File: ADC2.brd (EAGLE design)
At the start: 99.1 x 88.9 mm, 189 parts, among them IC1 FPGA CORE BOARD, IC10 REF5040, IC11 1.8V, IC12 1.8V, IC13 2.7V, IC14 ISO6720FB, IC15 ISO6720FB, IC16 IOS6720FB, IC17 IOS6720FB, IC2 OPA, IC3 7808, IC4 LM317-L, IC5 LM337-L, IC6 LM337-L, IC7 OPA1633, IC8 AK1110, IC9 AD4134, J1 V-, J2 V-, SW1 DC, SW2 GAIN, U1 DC-DC, X1 48MHz

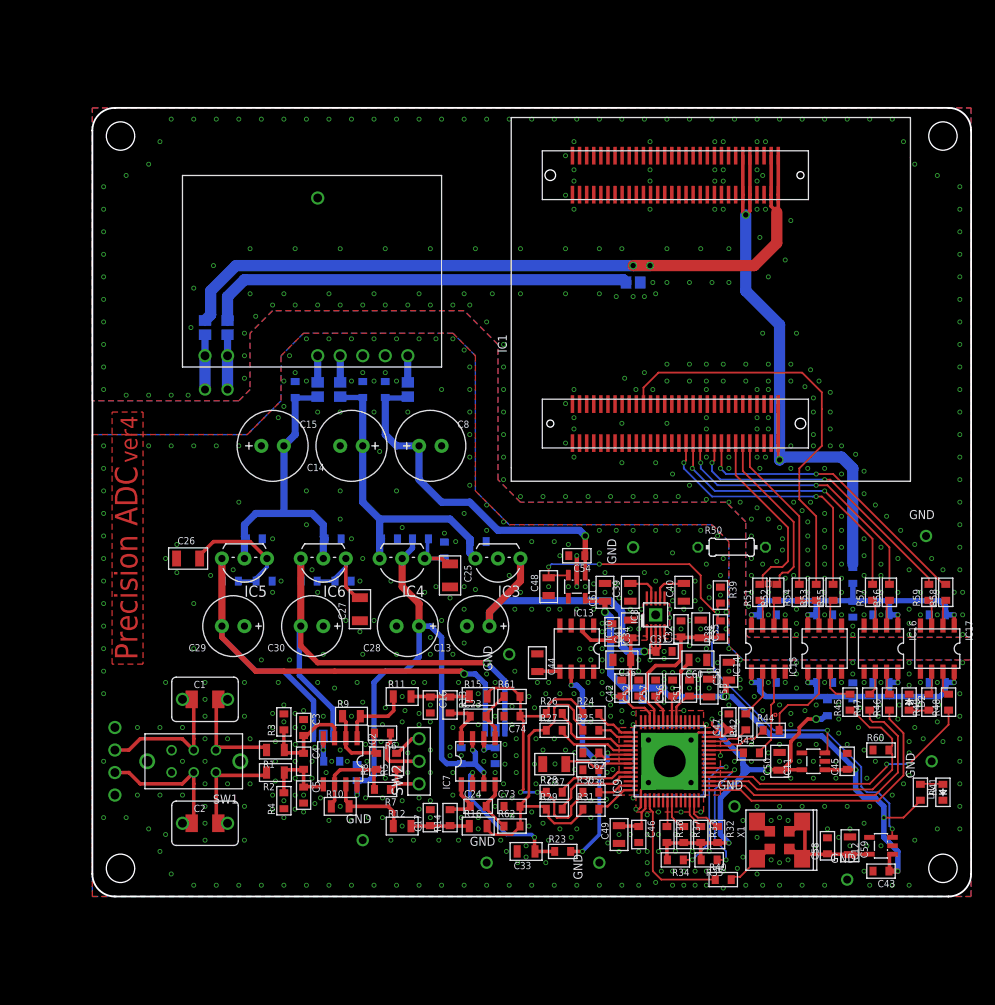
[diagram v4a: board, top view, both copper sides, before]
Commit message: 発注
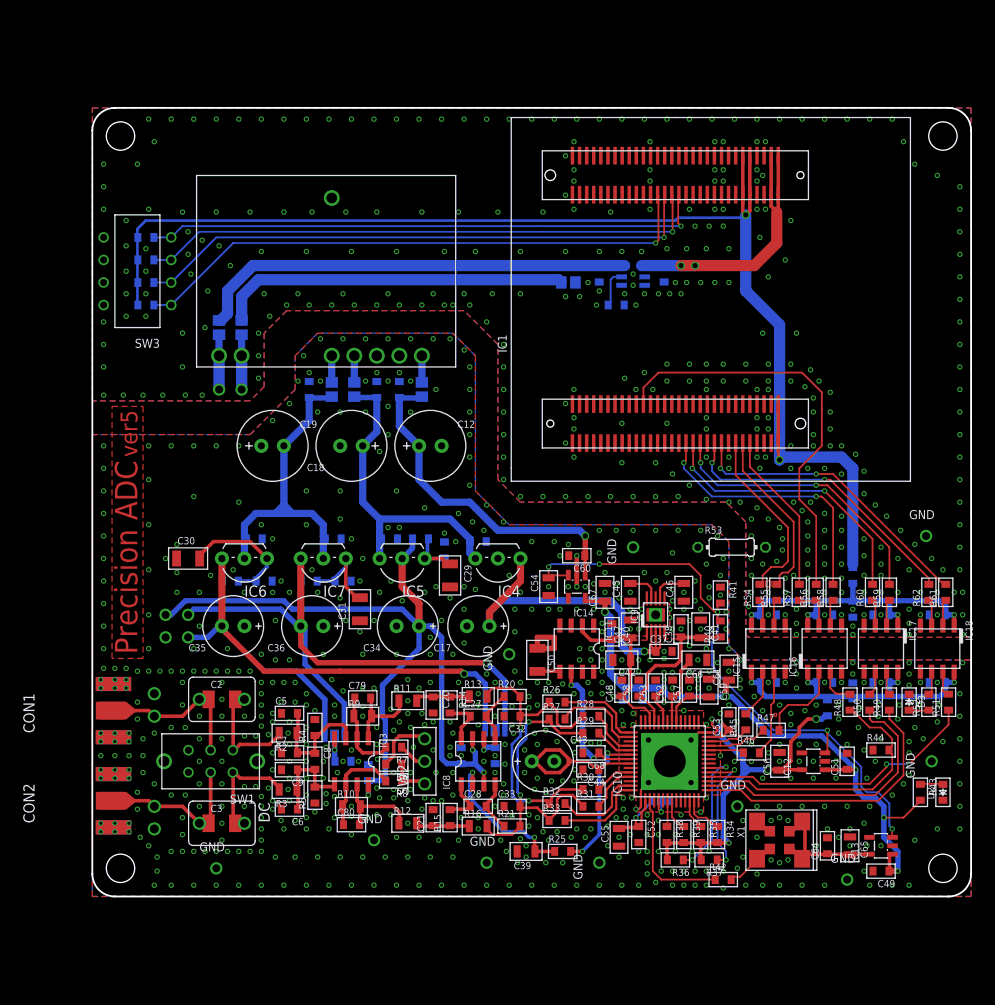
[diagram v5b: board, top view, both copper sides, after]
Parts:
- added C75, C76, C77: 0.1u, my_rcl:1608C
- added C78: 10u, my_rcl:1608C
- added C79, C80: 100p, my_rcl:1608C
- added CON1: IN-, my_connector:SMA-EDGE
- added CON2: IN+, my_connector:SMA-EDGE
- added IC18: IOS6720FB, my_ic:SOP8-2
- added J3: CLKSEL, my_rcl:1608-3-J
- added R63, R64, R65, R66: 10k, my_rcl:1608
- added SW3: FSEL, my_rcl:DIPSW-4
- added TP14, TP15: GND, my_connector:TESTPIN
- added TP16: +9V, my_connector:TESTPIN
- added TP17: -9V, my_connector:TESTPIN
- added TP18: -5V, my_connector:TESTPIN
- C1: device my_rcl:C050W -> my_rcl:1608C
- C10, C62: value 1u -> 0.1u
- C11, C38, C68: value 0.1u -> 1u
- C12, C18, C19: value 0.1u -> 100u; device my_rcl:1608C -> my_rcl:E2,5-8
- C13: value 100u -> 1u; device my_rcl:E2.5-6.5 -> my_rcl:1608C
- C14: value 100u -> 1u; device my_rcl:E2,5-8 -> my_rcl:1608C
- C15: value 100u -> 0.1u; device my_rcl:E2,5-8 -> my_rcl:1608C
- C16: value 1n -> 0.1u
- C17: value 1n -> 100u; device my_rcl:1608C -> my_rcl:E2.5-6.5
- C2: value 1u -> 1.5u
- C20, C21: value 0.1u -> 1n
- C23, C24: value 270p -> 0.1u
- C25, C26: value 10u -> 0.1u; device my_rcl:3216 -> my_rcl:1608C
- C27: value 10u -> 270p; device my_rcl:3216 -> my_rcl:1608C
- C28: value 100u -> 270p; device my_rcl:E2.5-6.5 -> my_rcl:1608C
- C29, C30: value 100u -> 10u; device my_rcl:E2.5-6.5 -> my_rcl:3216
- C3: value DNP -> 1.5u; device my_rcl:1608C -> my_rcl:C050W
- C31: value 1u -> 10u; device my_rcl:1608C -> my_rcl:3216
- C32: value 1u -> 68p
- C33: value 10u -> 68p; device my_rcl:2012 -> my_rcl:1608C
- C34: value 1u -> 100u; device my_rcl:1608C -> my_rcl:E2.5-6.5
- C35, C36: value 10u -> 100u; device my_rcl:2012 -> my_rcl:E2.5-6.5
- C37: value 10u -> 1u; device my_rcl:3216 -> my_rcl:1608C
- C4: value DNP -> 1u
- C40: value 10u -> 1u; device my_rcl:2012 -> my_rcl:1608C
- C42, C45, C46, C47, C54, C56, C65, C66, C67: value 0.1u -> 10u; device my_rcl:1608C -> my_rcl:2012
- C43: value 0.1u -> 330u; device my_rcl:1608C -> my_rcl:E2.5-6.5
- C44, C48, C49, C53, C60: value 10u -> 0.1u; device my_rcl:2012 -> my_rcl:1608C
- C50: device my_rcl:2012 -> my_rcl:3216
- C55: value 10u -> 2.2u
- C6: value 0.1u -> DNP
- C63, C72: value 10u -> 0.1u
- C69: value 0.1u -> 10u
- C7, C9: value 1u -> DNP
- C73, C74: value 47p -> 0.1u
- C8: value 100u -> DNP; device my_rcl:E2,5-8 -> my_rcl:1608C
- D1: value PWR -> TVS; device my_rcl:D1608 -> my_rcl:SOD323
- D2: value LED -> PWR
- D3: value TVS -> CLIP; device my_rcl:SOD323 -> my_rcl:D1608
- IC10: value REF5040 -> AD4134; device my_ic:SOP8 -> my_ic:QFN56-HT-HOLE
- IC11: value 1.8V -> REF5040; device my_ic:SOT23-5 -> my_ic:SOP8
- IC13: value 2.7V -> 1.8V
- IC14: value ISO6720FB -> 2.7V; device my_ic:SOP8 -> my_ic:SOT23-5
- IC15, IC17: device my_ic:SOP8 -> my_ic:SOP8-2
- IC16: value IOS6720FB -> ISO6720FB; device my_ic:SOP8 -> my_ic:SOP8-2
- IC2: value OPA -> AP22652; device my_ic:SOP8 -> my_ic:SOT23-6
- IC3: value 7808 -> OPA; device my_ic:TO-92 -> my_ic:SOP8
- IC4: value LM317-L -> 7808
- IC5: value LM337-L -> LM317-L
- IC7: value OPA1633 -> LM337-L; device my_ic:SOP8 -> my_ic:TO-92
- IC8: value AK1110 -> OPA1633; device my_ic:PLP10 -> my_ic:SOP8
- IC9: value AD4134 -> AK1110; device my_ic:QFN56-HT-HOLE -> my_ic:PLP10
- R1: value 10 -> 10k; device my_rcl:2012 -> my_rcl:1608
- R10, R9: value 1k -> 270
- R11, R12, R16: value 1k -> 510
- R13: value 360 -> 510; device my_rcl:1608 -> my_rcl:2012
- R14: value 360 -> 100
- R15: value 1k -> 100; device my_rcl:2012 -> my_rcl:1608
- R2: value 10 -> 20
- R20, R21: value 120 -> 51
- R24, R25: value 22 -> 120
- R26, R28, R29, R30, R31: value 22 -> 10; device my_rcl:1608 -> my_rcl:1608-3
- R27: value 22 -> 10
- R3: value 100k -> 20; device my_rcl:1608 -> my_rcl:2012
- R32: value 10k -> 10
- R33: value 10k -> 10; device my_rcl:1608 -> my_rcl:1608-3
- R38, R39: value 47k -> 10k
- R40: value 39 -> 47k
- R41: value 5.1k -> 47k
- R42: value ODR -> 39
- R43, R52: value DOUT -> 3.3k
- R44: value DCLK -> 10k
- R45: value SDO -> ODR
- R46: value CS -> DOUT
- R47, R57: value SCLK -> DCLK
- R48, R58: value SDI -> SDO
- R49, R59: value LED -> CS
- R5: value 360 -> 100k
- R50: value 10M -> SCLK; device my_rcl:0204/7 -> my_rcl:1608
- R51: value ODR -> SDI
- R53: value SUB -> 10M; device my_rcl:1608 -> my_rcl:0204/7
- R54: value DCLK -> ODR
- R55: value SDO -> DOUT
- R56: value CS -> SUB
- R6: value 10 -> 100
- R60: value 10k -> SCLK
- R61: value 50 -> SDI
- R62: value 50 -> LED
- R7: value 10 -> 24
- R8: value 10k -> 24
- SW1: value DC -> AC
- SW2: value GAIN -> GAIN H<>M
- moved C1 70.5 mm to (64.5, 70.2), flipped to the bottom, turned to 270 degrees
- moved C4 64.3 mm to (57.1, 70.2), flipped to the bottom
- moved IC2 63.8 mm to (61.0, 69.8), flipped to the bottom, turned to 270 degrees
- moved R1 63.2 mm to (59.1, 66.7), flipped to the bottom
- moved R62 53.9 mm to (94.3, 34.3), turned to 90 degrees
- moved C35 52.7 mm to (15.9, 30.5), turned to 180 degrees
- moved R61 50.3 mm to (96.2, 34.3), turned to 90 degrees
- moved C73 49.9 mm to (95.2, 24.1), flipped to the bottom
- moved R23 48.3 mm to (15.6, 35.6), flipped to the bottom
- moved IC13 45.0 mm to (88.9, 5.71), turned to 90 degrees
- moved C9 43.7 mm to (22.2, 14.3), flipped to the top, turned to 180 degrees
- moved C11 43.4 mm to (34.6, 57.1)
- moved C7 42.4 mm to (22.2, 16.2), flipped to the top, turned to 0 degrees
- moved R21 42.1 mm to (47.3, 7.94), flipped to the top
- moved C26 41.1 mm to (45.4, 15.9), flipped to the bottom, turned to 90 degrees
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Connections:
- removed net N$17 (its old number): IC14.6, R52.1
- new net DIPSW1: IC1.86, R63.1, SW3.1
- new net DIPSW2: IC1.88, R64.1, SW3.2
- new net DIPSW3: IC1.90, R65.1, SW3.3
- new net DIPSW4: IC1.92, R66.1, SW3.4
- new net N$32: IC16.6, R58.1
- new net N$57: IC10.47, J3.2
- new net N$63: IC2.5, R1.2
- new net VIN_LIM: C4.1, FB2.1, IC2.6
- net +1V8: now also C53.1, C56.1, IC10.13, IC12.5, R38.2, R39.2; no longer C47.1, C50.1, IC11.5, IC9.13, R32.2, R33.2
- net +1V8_ISO: now also C69.1, C70.1, C71.1, C72.1, C73.1, IC16.1, IC18.8; no longer C63.1, C64.1, C65.1, C66.1, C67.1, IC14.1, IC16.8
- net +3.6V: now also C11.1, C12.+, C60.1, IC14.1; no longer C54.1, C7.1, C8.+, IC13.1
- net +3V3D: now also R63.2, R64.2, R65.2, R66.2
- net +3V3D_ISO: now also C74.1, C75.1, C76.1, C77.1, C78.1, IC16.8, IC18.1; no longer C68.1, C69.1, C70.1, C71.1, C72.1, IC14.8, IC16.1
- net +5V: now also C38.1, C41.1, C58.1, IC10.25, IC9.5, R40.1; no longer C32.1, C35.1, C52.1, IC8.5, IC9.25, R38.1
- net +5V_DEL: now also C54.1, IC14.3, R40.2, R41.2; no longer C48.1, IC11.3, R38.2, R39.2
- net +8V: now also C17.+, C37.1, IC4.1, IC9.2, IC9.3, IC9.4; no longer C13.+, C31.1, IC3.1, IC8.2, IC8.3, IC8.4
- net +9V: now also C15.1, C25.1, C34.+, IC3.8, IC5.2, IC8.3, IC8.7, R22.2, TP16.1; no longer C11.1, C21.1, C28.+, IC2.8, IC4.2, IC7.3, IC7.7, R20.2
- net -5V: now also C36.-, IC7.3, R24.2, TP18.1; no longer C30.-, IC6.3, R22.2
- net -9V: now also C35.-, IC6.3, R23.2, TP17.1; no longer C29.-, IC5.3, R21.2
- net ADC+: now also C32.1, R13.2, R20.2, R32.1; no longer C74.1, R15.2, R24.1, R61.2
- net ADC-: now also C33.2, R21.2, R33.1; no longer C73.2, R25.1, R62.2
- net ADC_2V7: now also C49.1, C51.1, C63.1, C67.1, IC10.23, IC13.1, IC14.5, R43.2; no longer C43.1, C45.1, C55.1, C57.1, IC11.1, IC13.5, IC9.23, R41.2
- net ADC_AVDD1V8: now also C62.1, C66.1, IC10.21; no longer C56.1, C60.1, IC9.21
- net ADC_CLKVDD: now also C52.1, C55.1, IC10.44, J3.1; no longer C46.1, C49.1, IC9.44
- net ADC_CS: now also IC10.1, R49.1; no longer IC9.1, R46.1
- net ADC_DCLK: now also IC10.11, R47.1; no longer IC9.11, R44.1
- net ADC_DOUT: now also IC10.10, R46.1; no longer IC9.10, R43.1
- net ADC_DVDD1V8: now also C57.1, C59.1, IC10.20; no longer C51.1, C53.1, IC9.20
- net ADC_ODR: now also IC10.12, R45.1; no longer IC9.12, R42.1
- net ADC_SCLK: now also IC10.2, R50.1; no longer IC9.2, R47.1
- net ADC_SDI: now also IC10.4, R51.1; no longer IC9.4, R48.1
- net ADC_SDO: now also IC10.3, R44.2, R48.1; no longer IC9.3, R45.1, R60.2
- net ADC_VCOM: now also C39.2, IC8.2, R25.1; no longer C33.2, IC7.2, R23.1
- net AVDD5V: now also C40.1, C47.1, C48.1, D1.2, IC10.26, IC11.2, IC9.1; no longer C34.1, C36.1, C41.1, D3.2, IC10.2, IC8.1, IC9.26
- net DGND: now also C1.2, C4.2, C74.2, C75.2, C76.2, C77.2, C78.2, IC16.5, IC18.4, IC2.2, IC2.3, R1.1, R53.2, SW3.5, SW3.6, SW3.7, SW3.8; no longer C68.2, C69.2, C70.2, C71.2, C72.2, IC14.5, IC16.4, R50.2
- net FPGA_CS: now also R59.2; no longer R56.2
- net FPGA_DCLK: now also R57.2; no longer R54.2
- net FPGA_DCLK_SUB: now also R56.2; no longer R53.2
- net FPGA_DOUT: now also R55.2; no longer R52.2
- net FPGA_LED: now also R62.2; no longer R59.2
- net FPGA_ODR: now also R54.2; no longer R51.2
- net FPGA_SCLK: now also R60.2; no longer R57.2
- net FPGA_SDI: now also R61.2; no longer R58.2
- net FPGA_SDO: now also R58.2; no longer R55.2
- net GND: now also C10.2, C12.-, C13.2, C14.1, C15.2, C16.1, C17.-, C18.-, C19.+, C20.2, C22.2, C23.1, C24.1, C29.2, C30.1, C31.1, C34.-, C35.+, C36.+, C39.1, C43.-, C5.1, C68.2, C69.2, C7.1, C70.2, C71.2, C72.2, C73.2, CON1.G1, CON1.G2, CON1.G3, CON1.G4, CON2.G1, CON2.G2, CON2.G3, CON2.G4, D1.1, D3.K, IC10.14, IC10.19, IC10.22, IC10.24, IC10.27, IC10.31, IC10.37, IC10.40, IC10.43, IC10.HT, IC10.HT1, IC10.HT2, IC10.HT3, IC10.HT4, IC11.4, IC14.2, IC16.4, IC18.5, IC4.2, IC9.10, IC9.6, IC9.8, J3.3, R4.2, R41.1, R44.1, R5.1, R53.1, TP14.1, TP15.1; no longer C10.1, C12.1, C13.-, C14.-, C15.+, C16.2, C17.2, C18.2, C19.1, C20.1, C22.1, C27.1, C28.-, C29.+, C3.1, C30.+, C31.2, C34.2, C35.2, C36.2, C39.2, C43.2, C5.2, C7.2, C73.1, C74.2, C8.-, D1.K, D3.1, IC10.4, IC11.2, IC14.4, IC16.5, IC3.2, IC8.10, IC8.6, IC8.8, IC8.HT, IC9.14, IC9.19, IC9.22, IC9.24, IC9.27, IC9.31, IC9.37, IC9.40, IC9.43, IC9.47, IC9.HT1, IC9.HT3, IC9.HT4, R3.2, R39.1, R4.1, R50.1, R60.1
- net N$1: now also C80.1, IC3.6, R8.2; no longer IC2.6, R7.2, R8.1
- net N$10: now also IC16.2, R47.2; no longer IC15.2, R44.2
- net N$11: now also IC10.42, R33.2; no longer IC9.42, R31.2
- net N$12: now also C80.2, IC3.7; no longer IC2.7
- net N$13: now also IC10.41, R32.2; no longer IC9.41, R30.2
- net N$14: now also C5.2, C7.2, C8.1, IC3.3, R2.2, R4.1; no longer C3.2, C4.1, IC2.3, R1.2, R3.1
- net N$15: now also IC10.39, R31.2; no longer IC9.39, R29.2
- net N$16: now also IC16.3, R48.2; no longer IC15.3, R45.2
- net N$18: now also IC10.38, R30.2; no longer IC9.38, R28.2
- net N$19: now also C21.1, R15.1; no longer C17.1, R14.1
- net N$2: now also IC10.34, R25.2; no longer IC9.34, R23.2
- net N$20: now also IC10.33, R29.2; no longer IC9.33, R27.2
- net N$21: now also IC15.7, R54.1; no longer IC14.7, R51.1
- net N$22: now also C27.2, IC8.5, R20.1; no longer C23.2, IC7.5, R61.1
- net N$23: now also C6.1, C8.2, C9.1, IC3.5, R3.2, R5.2; no longer C4.2, C5.1, IC2.5, R2.2, R4.2
- net N$24: now also C27.1, IC8.8, R14.2; no longer C23.1, IC7.8, R13.2
- net N$25: now also IC10.32, R28.2; no longer IC9.32, R26.2
- net N$26: now also C28.1, IC8.1, R15.2; no longer C24.1, IC7.1, R14.2
- net N$27: now also IC16.7, R56.1, R57.1; no longer IC15.7, R53.1, R54.1
- net N$28: now also IC10.30, R27.2; no longer IC9.30, R25.2
- net N$29: now also IC10.29, R26.2; no longer IC9.29, R24.2
- net N$3: now also C79.1, IC3.2, R7.2; no longer IC2.2, R6.2, R8.2
- net N$30: now also R42.2; no longer R40.2
- net N$31: now also C28.2, IC8.4, R21.1; no longer C24.2, IC7.4, R62.1
- net N$33: now also IC17.6, R50.2; no longer IC16.6, R47.2
- net N$34: now also IC17.7, R49.2; no longer IC16.7, R46.2
- net N$35: now also IC18.6, R52.2; no longer IC17.6, R49.2
- net N$36: now also IC18.7, R51.2; no longer IC17.7, R48.2
- net N$37: now also IC17.3, R60.1; no longer IC16.3, R57.1
- net N$38: now also IC17.2, R59.1; no longer IC16.2, R56.1
- net N$39: now also IC18.3, R62.1; no longer IC17.3, R59.1
- net N$4: now also C79.2, IC3.1; no longer IC2.1
- net N$40: now also IC18.2, R61.1; no longer IC17.2, R58.1
- net N$41: now also C2.1, C2.3, CON1.SIG; no longer C1.1, C1.3
- net N$42: now also C3.1, C3.3, CON2.SIG; no longer C2.1, C2.3
- net N$43: now also C2.2, C2.4, R2.1; no longer C1.2, C1.4, R1.1
- net N$44: now also C3.2, C3.4, R3.1; no longer C2.2, C2.4, R2.1
- net N$45: now also R7.1; no longer R6.1
- net N$46: now also R6.1, R8.1; no longer R5.1, R7.1
- net N$47: now also D3.A, R52.1; no longer D2.A, R49.1
- net N$48: now also C50.1, IC11.5; no longer C44.1, IC10.5
- net N$49: now also IC10.5, R37.1; no longer IC9.5, R35.1
- net N$5: now also C20.1, R14.1; no longer C16.1, R15.1
- net N$50: now also IC10.6, R36.1; no longer IC9.6, R34.1
- net N$52: now also C16.2, IC3.4; no longer C12.2, IC2.4
- net N$53: now also C29.1, IC5.1, R22.1; no longer C25.1, IC4.1, R20.1
- net N$54: now also C30.2, IC6.1, R23.1; no longer C26.2, IC5.1, R21.1
- net N$55: now also C31.2, IC7.1, R24.1; no longer C27.2, IC6.1, R22.1
- net N$58: now also D2.A, R43.1; no longer D1.A, R41.1
- net N$59: now also R6.2; no longer R5.2
- net N$6: now also C45.1, IC9.9; no longer C39.1, IC8.9
- net N$60: now also IC10.50, R39.1; no longer IC9.50, R37.1
- net N$61: now also IC10.55, R34.1; no longer IC9.55, R32.1
- net N$62: now also IC10.54, R35.1; no longer IC9.54, R33.1
- net N$64: now also IC10.49, R38.1; no longer IC9.49, R36.1
- net N$7: now also C46.1, IC9.7; no longer C40.1, IC8.7
- net N$74: now also C26.2, IC8.6; no longer C22.2, IC7.6
- net N$8: now also IC15.2, R45.2; no longer IC14.2, R42.2
- net N$9: now also IC15.3, R46.2; no longer IC14.3, R43.2
- net OSC_CLK: now also IC10.45, R42.1; no longer IC9.45, R40.1
- net V+: now also C10.1, C13.1, C18.+, C22.1, IC5.3; no longer C14.+, C18.1, C6.1, C9.1, IC3.3
- net V-: now also C14.2, C19.-, C23.2, C24.2, IC7.2; no longer C10.2, C15.-, C19.2, C20.2, IC5.2
- net VCC_OSC: now also C64.1, C65.1, IC13.5; no longer C58.1, C59.1, IC12.5
- net VIN: now also C1.1, IC2.1; no longer FB2.1
- net VREF: now also C68.1, IC10.35, IC11.6; no longer C62.1, IC10.6, IC9.35
- net VREFCAP: now also C43.+, C44.1, IC10.36; no longer C37.1, C38.1, IC9.36
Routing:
- net +3V3D: track 69.3 -> 147.3 mm
- net DIPSW1: track 0.00 -> 65.1 mm, vias 0 -> 1
- net DIPSW2: track 0.00 -> 64.5 mm, vias 0 -> 1
- net DIPSW3: track 0.00 -> 64.0 mm, vias 0 -> 1
- net DIPSW4: track 0.00 -> 63.7 mm, vias 0 -> 1
- net VIN: track 88.1 -> 34.9 mm
- net VIN_LIM: track 0.00 -> 50.3 mm
- net +9V: track 62.9 -> 91.7 mm
- net -5V: track 56.6 -> 70.8 mm
- net VREFCAP: track 8.13 -> 18.7 mm
- net N$56: track 48.5 -> 39.6 mm
- net N$28: track 3.90 -> 10.4 mm
- net N$13: track 3.90 -> 10.2 mm
- net N$11: track 4.48 -> 9.75 mm
- net N$29: track 4.63 -> 9.75 mm
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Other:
- board text added: "DC"
- board text added: "ver5"
- board text removed: "ver4"

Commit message: 入力回路変更
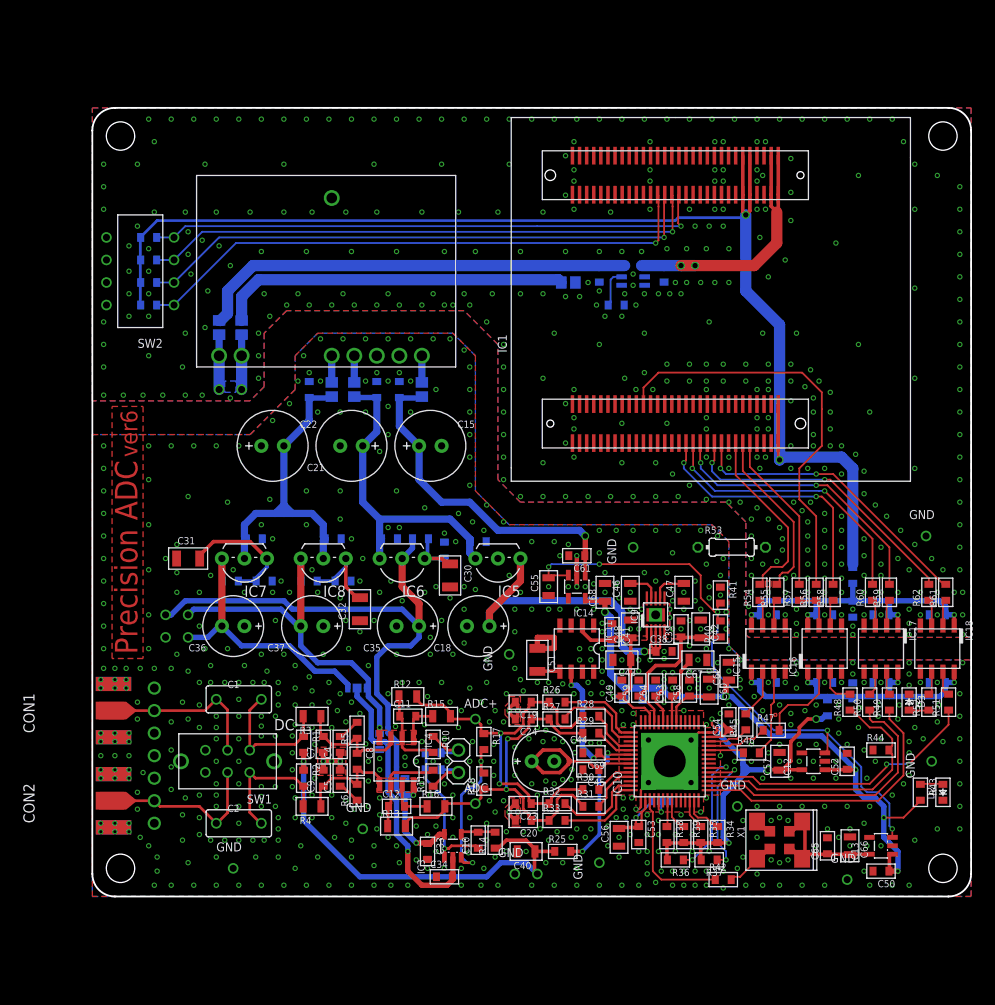
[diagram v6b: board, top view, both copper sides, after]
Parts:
- removed C80: 100p, my_rcl:1608C
- removed J3: CLKSEL, my_rcl:1608-3-J
- removed SW3: FSEL, my_rcl:DIPSW-4
- added JP1: GAIN, my_connector:1X02
- added TP19, TP20, TP21: GND, my_connector:TESTPIN-MID
- added TP22: VCOM, my_connector:TESTPIN
- added TP23: ADC+, my_connector:TESTPIN
- added TP24: ADC-, my_connector:TESTPIN
- C1: value 1u -> 1.5u; device my_rcl:1608C -> my_rcl:C050
- C10: value 0.1u -> 68p; device my_rcl:1608C -> my_rcl:1608-3
- C11: value 1u -> 100p
- C12: value 100u -> 100p; device my_rcl:E2,5-8 -> my_rcl:1608C
- C13: value 1u -> 0.1u
- C15, C22: value 0.1u -> 100u; device my_rcl:1608C -> my_rcl:E2,5-8
- C16: value 0.1u -> 1u
- C17: value 100u -> 1u; device my_rcl:E2.5-6.5 -> my_rcl:1608C
- C18: device my_rcl:E2,5-8 -> my_rcl:E2.5-6.5
- C19: value 100u -> 100p; device my_rcl:E2,5-8 -> my_rcl:1608-3
- C2: device my_rcl:C050W -> my_rcl:C050
- C20: value 1n -> 100p; device my_rcl:1608C -> my_rcl:1608-3
- C21: value 1n -> 100u; device my_rcl:1608C -> my_rcl:E2,5-8
- C23, C24: value 0.1u -> 100p
- C27, C28: value 270p -> 0.1u
- C29, C50: value 10u -> 0.1u; device my_rcl:3216 -> my_rcl:1608C
- C3: value 1.5u -> 1u; device my_rcl:C050W -> my_rcl:1608C
- C32: value 68p -> 10u; device my_rcl:1608C -> my_rcl:3216
- C33: value 68p -> 0.1u
- C34: value 100u -> 0.1u; device my_rcl:E2.5-6.5 -> my_rcl:1608C
- C37: value 1u -> 100u; device my_rcl:1608C -> my_rcl:E2.5-6.5
- C39, C41: value 10u -> 1u; device my_rcl:2012 -> my_rcl:1608C
- C4: value 1u -> 22p
- C40, C68: value 1u -> 10u; device my_rcl:1608C -> my_rcl:2012
- C43: value 330u -> 10u; device my_rcl:E2.5-6.5 -> my_rcl:2012
- C44: value 0.1u -> 330u; device my_rcl:1608C -> my_rcl:E2.5-6.5
- C45, C54, C59, C61, C65: value 10u -> 0.1u; device my_rcl:2012 -> my_rcl:1608C
- C48, C57, C60, C62: value 0.1u -> 10u; device my_rcl:1608C -> my_rcl:2012
- C5: value DNP -> 22p
- C51: value 0.1u -> 10u; device my_rcl:1608C -> my_rcl:3216
- C55: value 2.2u -> 10u
- C56: value 10u -> 2.2u
- C6: value DNP -> 1u
- C69: value 10u -> 1u
- C70: value 0.1u -> 10u
- C78: value 10u -> 0.1u
- C79: value 100p -> 10u
- C8: device my_rcl:1608C -> my_rcl:1608-3
- IC15, IC16: value ISO6720FB -> SI8620
- IC17, IC18: value IOS6720FB -> SI8620
- IC3: device my_ic:SOP8 -> my_ic:SOT23-5
- IC4: value 7808 -> OPA; device my_ic:TO-92 -> my_ic:SOP8
- IC5: value LM317-L -> 7808
- IC6: value LM337-L -> LM317-L
- IC8: value OPA1633 -> LM337-L; device my_ic:SOP8 -> my_ic:TO-92
- J1: value V- -> V-SEL; device my_rcl:2012-3-J -> my_rcl:1608-3-J
- J2: value V- -> CLKSEL; device my_rcl:2012-3-J -> my_rcl:1608-3-J
- R1: value 10k -> 100k; device my_rcl:1608 -> my_rcl:1608-3
- R10: value 270 -> 24; device my_rcl:2012 -> my_rcl:1608-3
- R11: value 510 -> 24; device my_rcl:2012 -> my_rcl:1608-3
- R12, R13, R3: device my_rcl:2012 -> my_rcl:2012-R
- R14: value 100 -> 1k
- R15: value 100 -> 270; device my_rcl:1608 -> my_rcl:2012-R
- R16: value 510 -> 270; device my_rcl:2012 -> my_rcl:2012-R
- R17, R18: value 680 -> 3.6k
- R19: value 330 -> 680
- R2: value 20 -> 100k; device my_rcl:2012 -> my_rcl:1608-3
- R20: value 51 -> 680
- R21: value 51 -> 330
- R4: value 100k -> 20; device my_rcl:1608 -> my_rcl:2012-R
- R5: value 100k -> 50; device my_rcl:1608 -> my_rcl:1608-3
- R6: value 100 -> 50; device my_rcl:1608 -> my_rcl:1608-3
- R7: value 24 -> 10k
- R8: value 24 -> 1k; device my_rcl:1608 -> my_rcl:1608-3
- R9: value 270 -> 1k; device my_rcl:2012 -> my_rcl:1608-3
- SW2: value GAIN H<>M -> MODE-SW; device my_connector:1X03 -> my_rcl:DIPSW-4
- moved C3 79.5 mm to (64.5, 70.2), flipped to the bottom, turned to 270 degrees
- moved C6 69.7 mm to (57.1, 70.2), flipped to the bottom, turned to 270 degrees
- moved C1 67.8 mm to (16.5, 22.2), flipped to the top, turned to 0 degrees
- moved SW2 63.9 mm to (5.40, 70.5)
- moved R1 60.8 mm to (23.8, 17.1), flipped to the top, turned to 270 degrees
- moved C4 60.5 mm to (27.9, 17.1), flipped to the top, turned to 90 degrees
- moved C79 56.1 mm to (85.7, 32.4), flipped to the bottom, turned to 270 degrees
- moved R7 55.8 mm to (59.1, 66.7), flipped to the bottom, turned to 0 degrees
- moved C50 45.5 mm to (88.9, 2.86), turned to 180 degrees
- moved C21 42.9 mm to (29.2, 50.8), turned to 180 degrees
- moved C23 42.5 mm to (48.6, 10.5), flipped to the top, turned to 180 degrees
- moved C16 42.1 mm to (32.1, 57.1), turned to 90 degrees
- moved C12 40.8 mm to (34.3, 10.2)
- moved C19 40.4 mm to (48.6, 21.9), turned to 180 degrees
- moved C37 39.8 mm to (24.8, 30.5), turned to 180 degrees
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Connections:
- removed net N$26: C28.1, IC8.1, R15.2
- removed net N$59: R6.2, SW2.3
- removed net N$74: C26.2, IC8.6, J2.2
- net +1V8: now also C54.1, C57.1; no longer C53.1, C56.1
- net +1V8_ISO: now also C74.1; no longer C69.1
- net +3.6V: now also C14.1, C15.+, C61.1; no longer C11.1, C12.+, C60.1
- net +3V3D_ISO: now also C79.1; no longer C74.1
- net +5V: now also C39.1, C42.1, C59.1; no longer C38.1, C41.1, C58.1
- net +5V_DEL: now also C55.1; no longer C54.1
- net +8V: now also C18.+, C38.1, IC5.1; no longer C17.+, C37.1, IC4.1
- net +9V: now also C28.1, C33.1, C35.+, IC3.5, IC4.8, IC6.2; no longer C15.1, C25.1, C34.+, IC3.8, IC5.2, IC8.3, IC8.7
- net -5V: now also C29.2, C37.-, IC4.4, IC8.3, J1.3; no longer C36.-, IC7.3, J1.1, J2.1
- net -9V: now also C36.-, IC7.3, J1.1; no longer C35.-, IC6.3, J1.3, J2.3
- net ADC+: now also C19.1, C23.1, R12.2, R15.2, R17.1, TP23.1; no longer C32.1, R13.2, R20.2
- net ADC-: now also C20.1, C24.1, R13.2, R18.1, TP24.1; no longer C33.2, R21.2
- net ADC_2V7: now also C50.1, C52.1, C62.1, C64.1, C68.1; no longer C49.1, C51.1, C61.1, C63.1, C67.1
- net ADC_AVDD1V8: now also C63.1, C67.1; no longer C62.1, C66.1
- net ADC_CLKVDD: now also C53.1, C56.1, J2.1; no longer C52.1, C55.1, J3.1
- net ADC_DVDD1V8: now also C58.1, C60.1; no longer C57.1, C59.1
- net ADC_VCOM: now also C40.2, R1.2, R14.1, R2.1, TP22.1; no longer C39.2, IC8.2
- net AVDD5V: now also C41.1, C43.1, C49.1; no longer C40.1, C42.1, C47.1
- net DGND: now also C3.2, C6.2, C79.2, R7.1, SW2.5, SW2.6, SW2.7, SW2.8; no longer C1.2, C4.2, C74.2, R1.1, SW3.5, SW3.6, SW3.7, SW3.8
- net DIPSW1: now also SW2.1; no longer SW3.1
- net DIPSW2: now also SW2.2; no longer SW3.2
- net DIPSW3: now also SW2.3; no longer SW3.3
- net DIPSW4: now also SW2.4; no longer SW3.4
- net GND: now also C14.2, C15.-, C16.2, C17.1, C19.2, C21.-, C22.+, C23.2, C24.2, C27.1, C28.2, C29.1, C30.2, C32.1, C33.2, C34.1, C35.-, C37.+, C39.2, C4.1, C40.1, C43.2, C44.-, C5.2, C74.2, IC5.2, J2.3, R19.1, R20.2, R21.2, TP19.1, TP20.1, TP21.1; no longer C10.2, C11.2, C12.-, C14.1, C15.2, C16.1, C17.-, C19.+, C21.2, C22.2, C23.1, C24.1, C29.2, C30.1, C32.2, C33.1, C34.-, C35.+, C37.2, C39.1, C40.2, C43.-, C44.2, C5.1, C6.2, IC4.2, J3.3, R17.1, R18.2, R19.2, R4.2, R5.1
- net N$1: now also C12.1, IC4.6, R11.2, R13.1; no longer C80.1, IC3.6, R10.1, R8.2
- net N$12: now also C5.1, R6.1; no longer C80.2, IC3.7, R10.2, R12.1
- net N$14: now also IC4.3, R3.2, R5.1; no longer C5.2, IC3.3, R2.2, R4.1
- net N$19: now also IC3.3, R17.2, R18.2; no longer C21.1, R12.2, R15.1, R16.1
- net N$22: now also C10.2, IC3.4, R14.2; no longer C27.2, IC8.5, R20.1
- net N$23: now also IC4.5, R4.2, R6.2; no longer C6.1, IC3.5, R3.2, R5.2
- net N$24: now also C34.2, IC3.2, J1.2; no longer C27.1, IC8.8, R14.2
- net N$3: now also C11.1, IC4.2, R10.2, R12.1; no longer C79.1, IC3.2, R7.2, R9.1
- net N$31: now also C11.2, IC4.1, R15.1; no longer C28.2, IC8.4, R21.1
- net N$4: now also C4.2, R5.2; no longer C79.2, IC3.1, R11.1, R9.2
- net N$41: now also C1.1; no longer C2.1, C2.3
- net N$42: now also C2.1; no longer C3.1, C3.3
- net N$43: now also C1.2, R1.1, R3.1; no longer C2.2, C2.4, R2.1
- net N$44: now also C2.2, R2.2, R4.1; no longer C3.2, C3.4, R3.1
- net N$45: now also JP1.1, R10.1, R8.1; no longer R7.1, SW2.2
- net N$46: now also JP1.2, R11.1, R9.1; no longer R6.1, R8.1, SW2.1
- net N$48: now also C51.1; no longer C50.1
- net N$5: now also C10.1, IC3.1, R8.2, R9.2; no longer C20.1, R11.2, R13.1, R14.1
- net N$52: now also C12.2, IC4.7, R16.1; no longer C16.2, IC3.4, J1.2
- net N$53: now also C30.1, IC6.1, R19.2; no longer C29.1, IC5.1, R17.2
- net N$54: now also C31.2, IC7.1, R20.1; no longer C30.2, IC6.1, R18.1
- net N$55: now also C32.2, IC8.1, R21.1; no longer C31.2, IC7.1, R19.1
- net N$57: now also J2.2; no longer J3.2
- net N$6: now also C46.1; no longer C45.1
- net N$63: now also R7.2; no longer R1.2
- net N$7: now also C47.1; no longer C46.1
- net V+: now also C16.1, C21.+, C25.1, IC6.3; no longer C10.1, C18.+, C22.1, IC4.3
- net V-: now also C17.2, C22.-, C26.2, C27.2, IC8.2; no longer C14.2, C19.-, C23.2, C24.2, IC6.2
- net VCC_OSC: now also C66.1; no longer C64.1
- net VIN: now also C3.1; no longer C1.1
- net VIN_LIM: now also C6.1; no longer C4.1
- net VREF: now also C69.1; no longer C68.1
- net VREFCAP: now also C44.+, C45.1; no longer C43.+, C44.1
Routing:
- net -9V: track 71.7 -> 31.8 mm, vias 1 -> 0
- net ADC_VCOM: track 17.3 -> 49.3 mm, vias 2 -> 1
- net -5V: track 70.8 -> 43.4 mm
- net N$24: track 5.40 -> 32.3 mm, vias 0 -> 1
- net GND: track 18.5 -> 33.7 mm, vias 684 -> 663
- net +9V: track 91.7 -> 77.4 mm, vias 3 -> 2
- net N$19: track 6.34 -> 18.2 mm, vias 0 -> 2
- net N$5: track 6.57 -> 17.0 mm, vias 0 -> 1
- net ADC-: track 34.8 -> 44.3 mm
- net N$12: track 10.7 -> 2.56 mm
- net ADC+: track 36.0 -> 43.9 mm
- net N$59: track 6.80 -> 0.00 mm
- net N$4: track 9.29 -> 2.56 mm
- net N$26: track 5.32 -> 0.00 mm
- net N$74: track 4.71 -> 0.00 mm, vias 1 -> 0
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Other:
- board text added: "ver6"
- board text removed: "ver5"

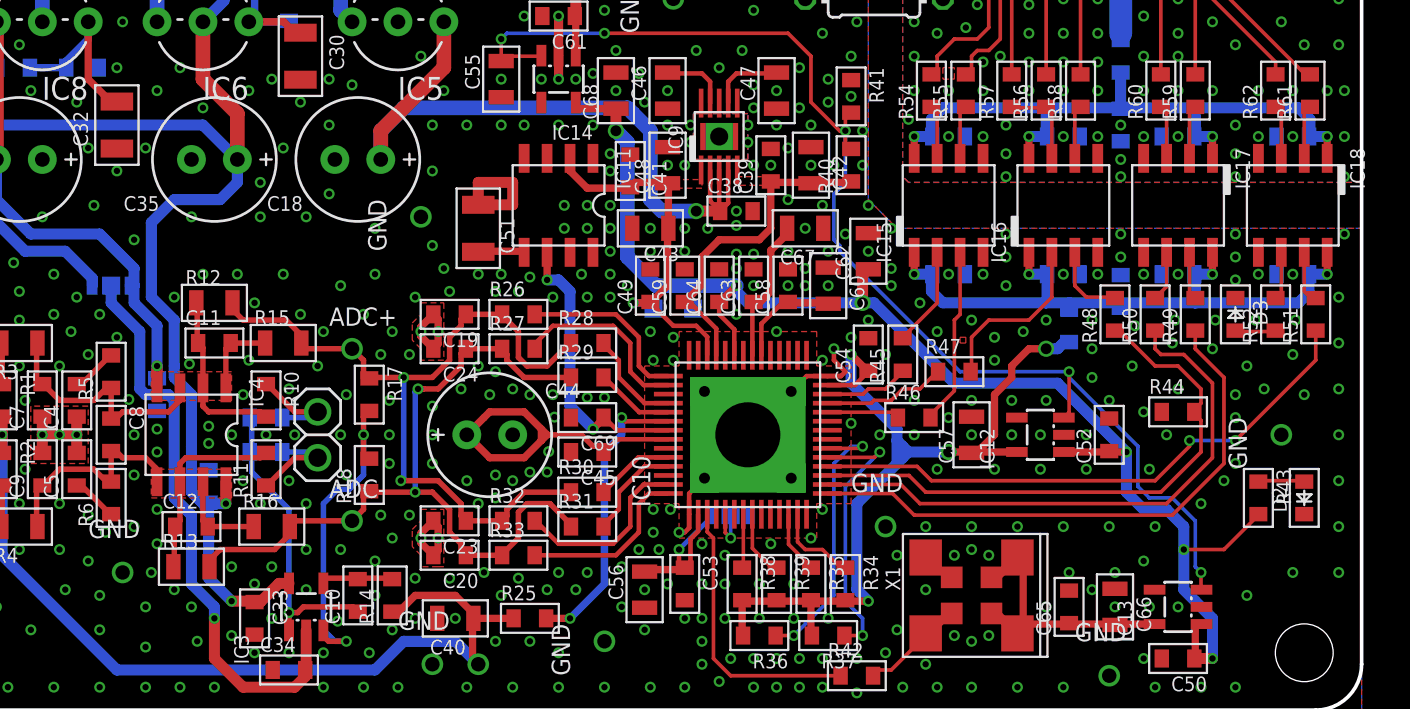
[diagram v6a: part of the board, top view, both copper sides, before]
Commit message: 6層
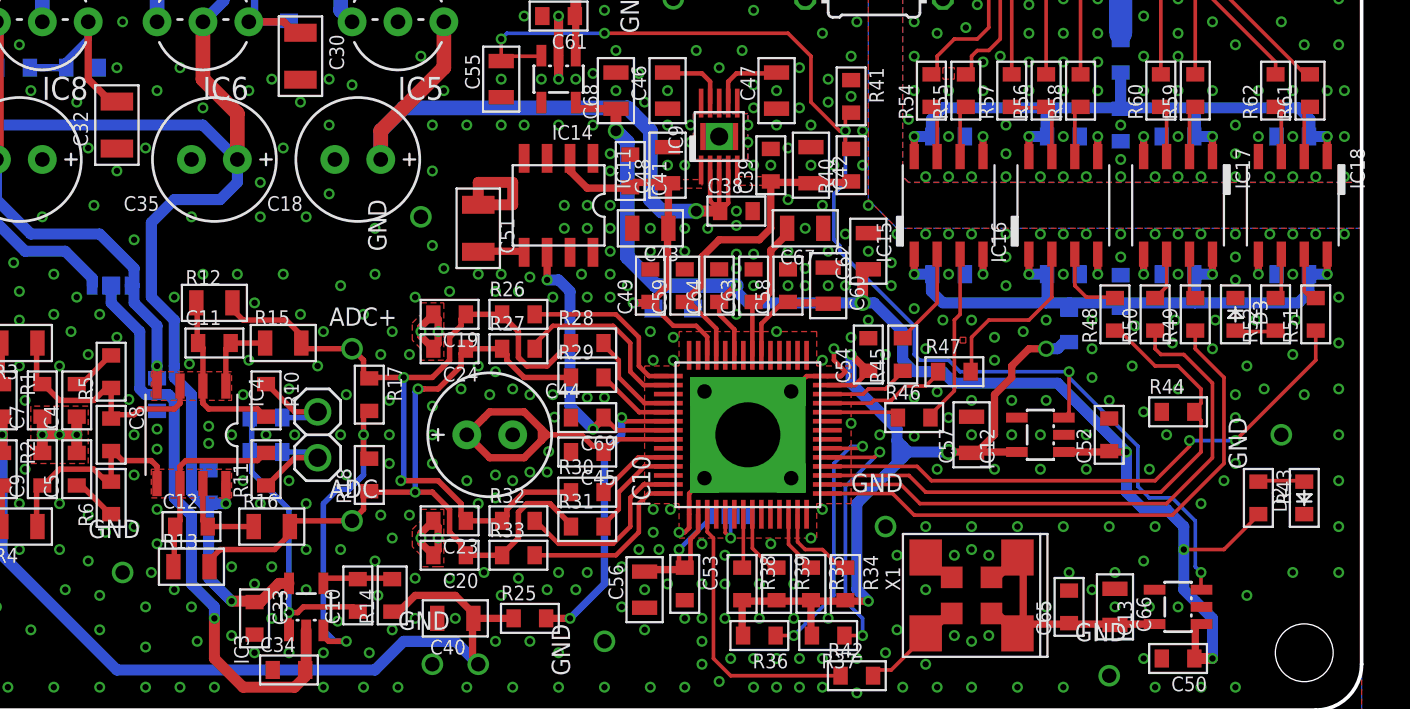
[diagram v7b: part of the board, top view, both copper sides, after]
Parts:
- IC4: device my_ic:SOP8 -> my_ic:SOP8-3
- R45, R46: device my_rcl:1608 -> my_rcl:1608-3
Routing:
- net GND: track 33.7 -> 38.1 mm, vias 663 -> 678
- net DGND: track 0.00 -> 3.33 mm, vias 380 -> 392
- net ADC_2V7: track 75.8 -> 76.7 mm
- net +5V_DEL: track 69.8 -> 70.7 mm
- added copper zone on layer 14, net DGND
- added copper zone on layer 3, net DGND
- added copper zone on layer 14, net GND
- added copper zone on layer 3, net GND
